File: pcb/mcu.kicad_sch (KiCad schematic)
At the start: 35 parts, among them J1 XF2M-1415-1A, SW1 EVQ-Q2B02W, SW2 EVQ-Q2B02W, U1 ESP32-S3-WROOM-1-N8R2

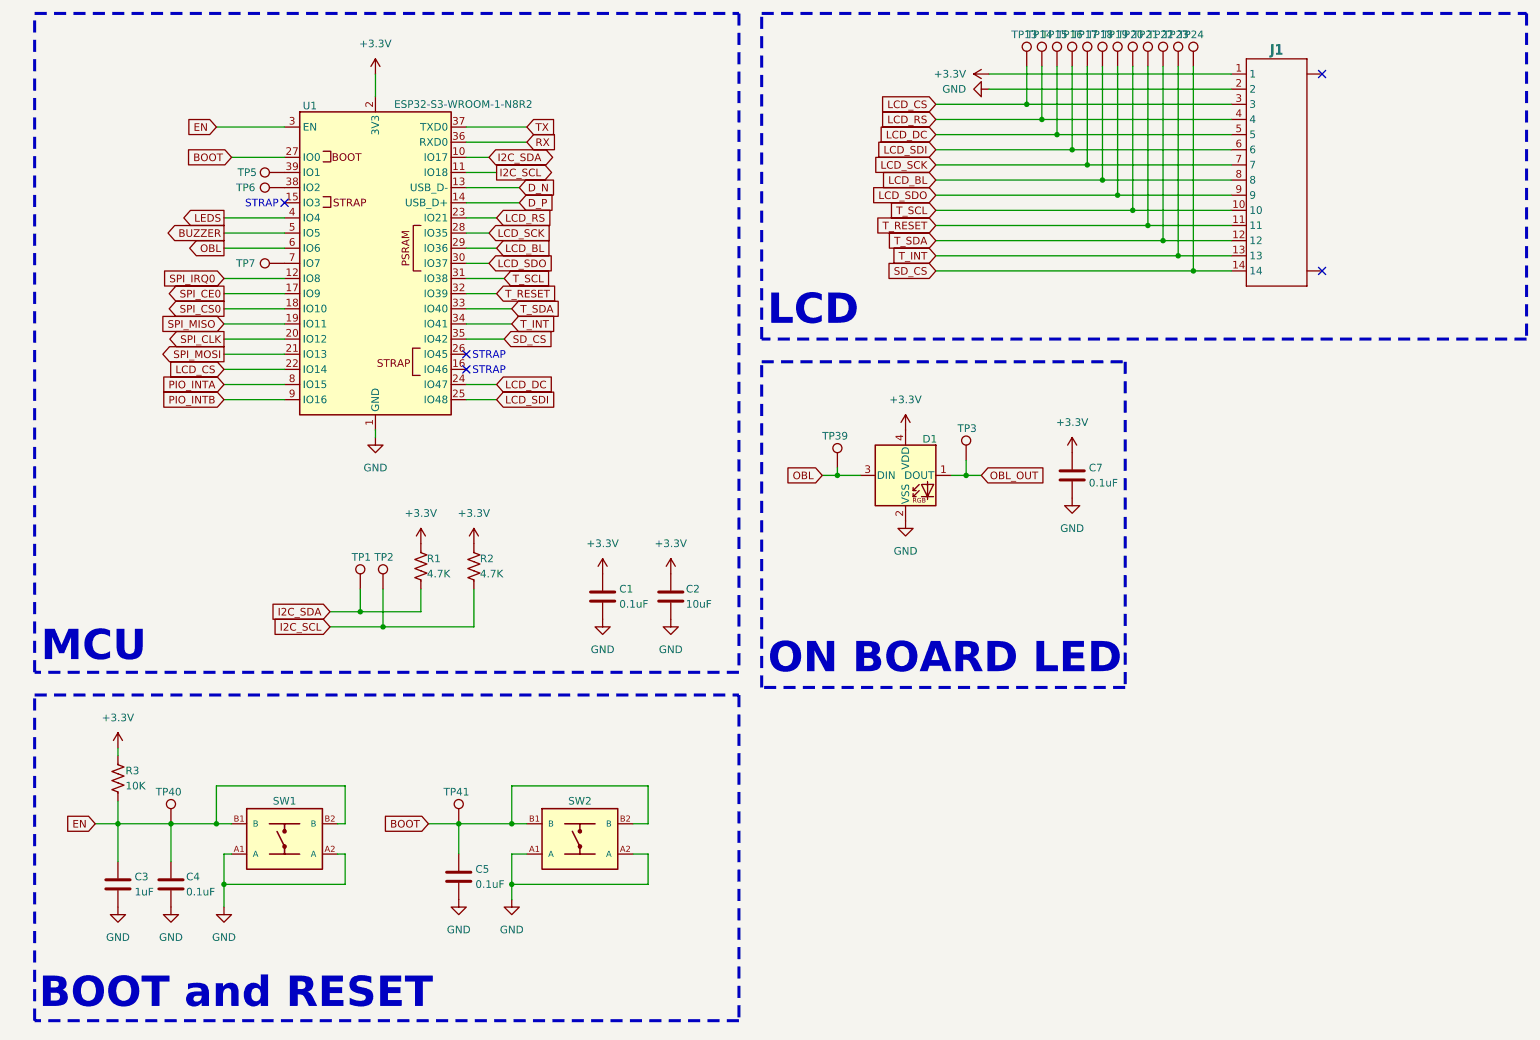
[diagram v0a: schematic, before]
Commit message: Clean up and consistency
Moved buzzer to MCU
Fixed model directory
Set font size
Set outline size
Upscaled Roxy ❤️
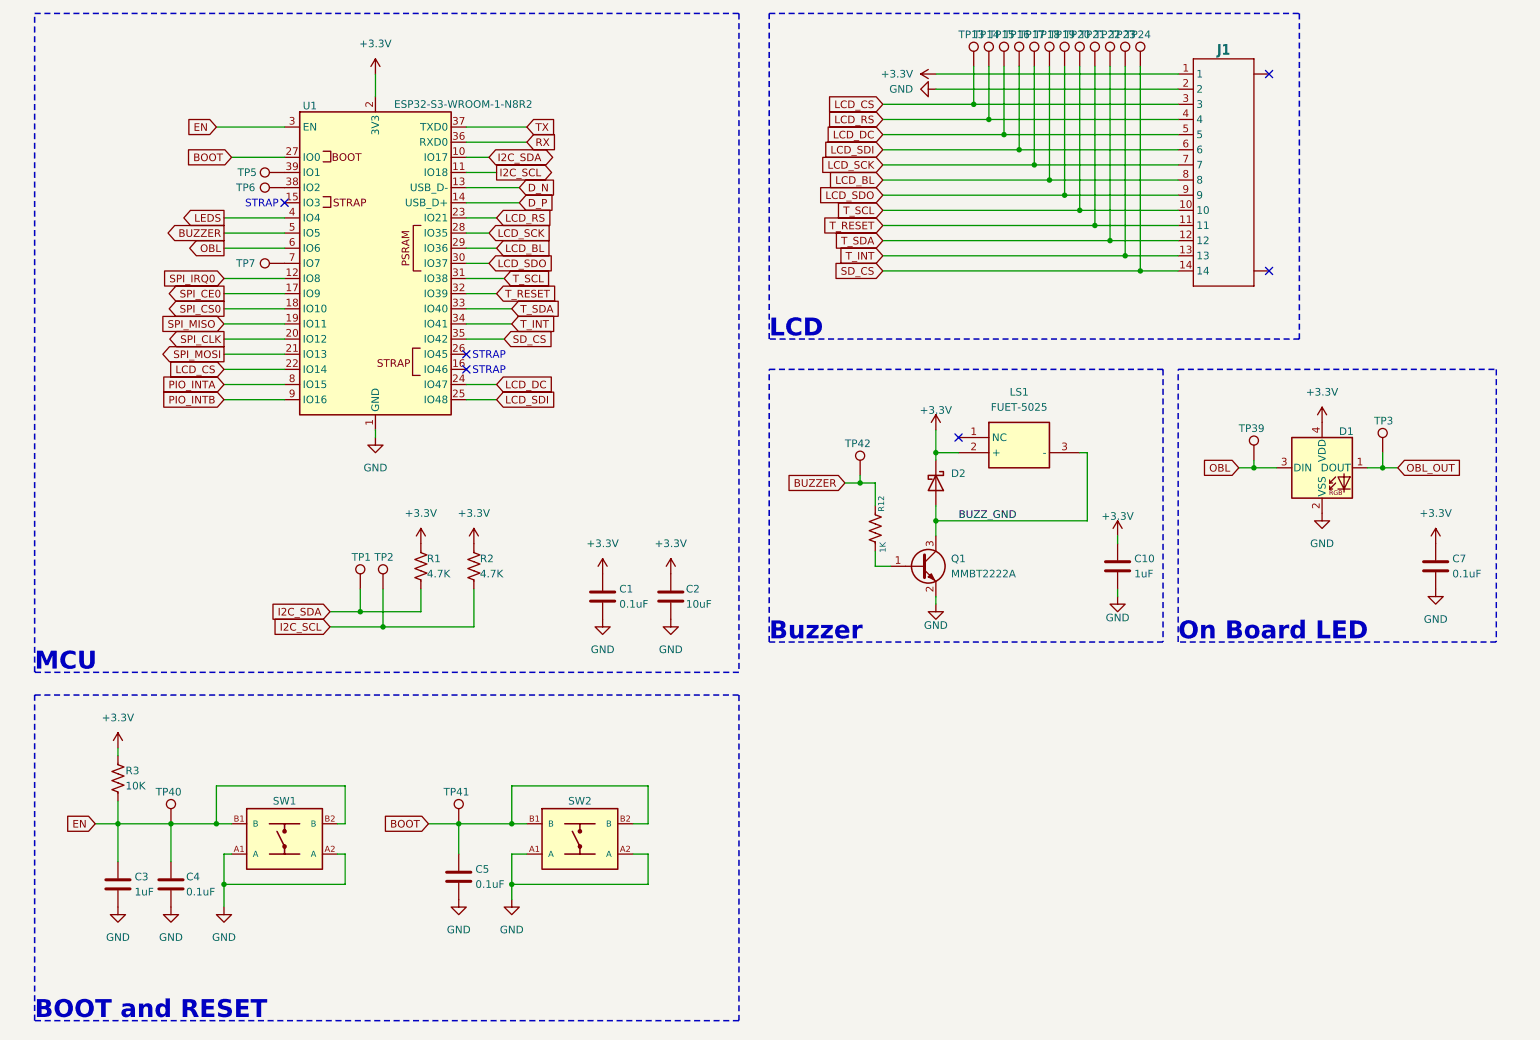
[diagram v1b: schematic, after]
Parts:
- added C10: 1uF, CRGM Passive:C_0603_1608Metric, symbol Device:C
- added D2: D_Schottky, CRGM Passive:D_SOD-523, symbol Device:D_Schottky
- added LS1: FUET-5025, CRG Makes:FUET-5025, symbol CRG Makes:CMT-0502-75-SMT-TR
- added Q1: MMBT2222A, CRGM Passive:SOT-523, symbol Transistor_BJT:MMBT2222A
- added R12: 1K, CRGM Passive:R_0603_1608Metric, symbol Device:R_US
- added TP42: ~, CRGM Mechanical:TestPoint_Pad_D1.0mm, symbol Connector:TestPoint
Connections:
- net +3.3V: now also C10.1, D2.1 (K), LS1.2 (+)
- net BUZZER: now also R12.1, TP42.1
- net GND: now also C10.2, Q1.2 (E)
- new net: Q1.1 (B), R12.2
- new net BUZZ_GND: D2.2 (A), LS1.3 (-), Q1.3 (C)
- no-connect marks 5 -> 6
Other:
- note added: "Buzzer"
- note added: "On Board LED"
- note removed: "ON BOARD LED"
- moved on the sheet: C7, D1, J1, TP13, TP14, TP15, TP16, TP17, TP18, TP19, TP20, TP21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
